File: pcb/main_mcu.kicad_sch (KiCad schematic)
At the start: 16 parts, among them U3 STM32H563VITx

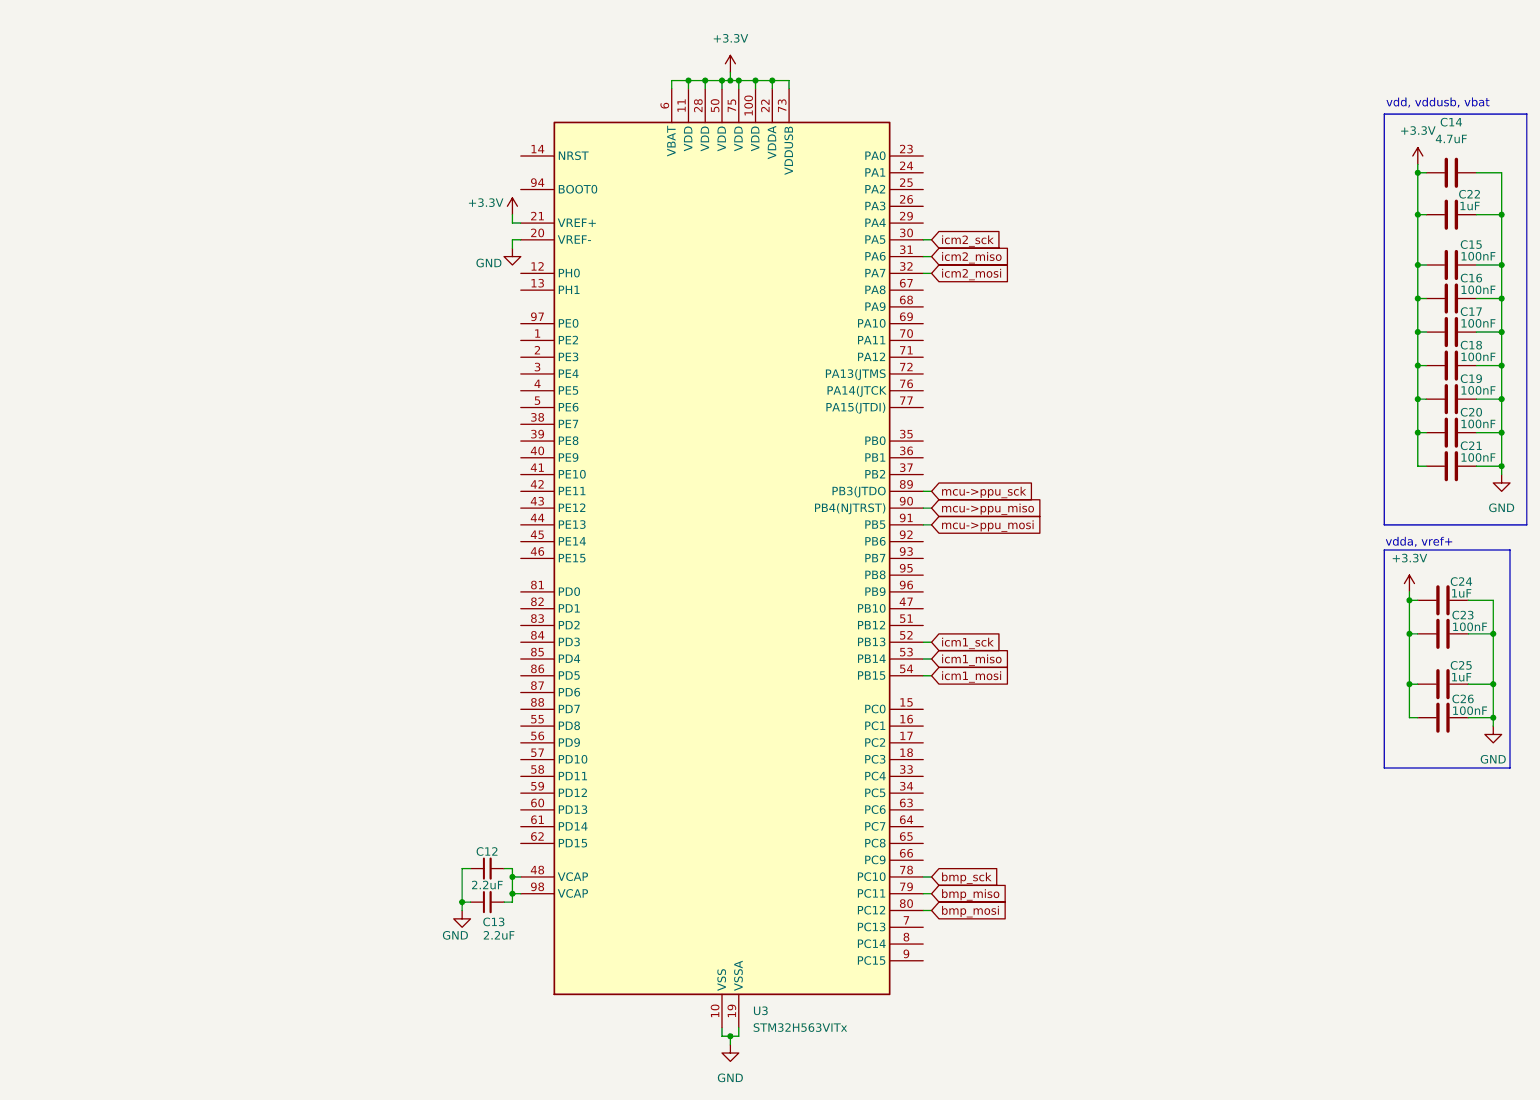
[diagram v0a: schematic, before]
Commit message: tons of work on rf and mcu
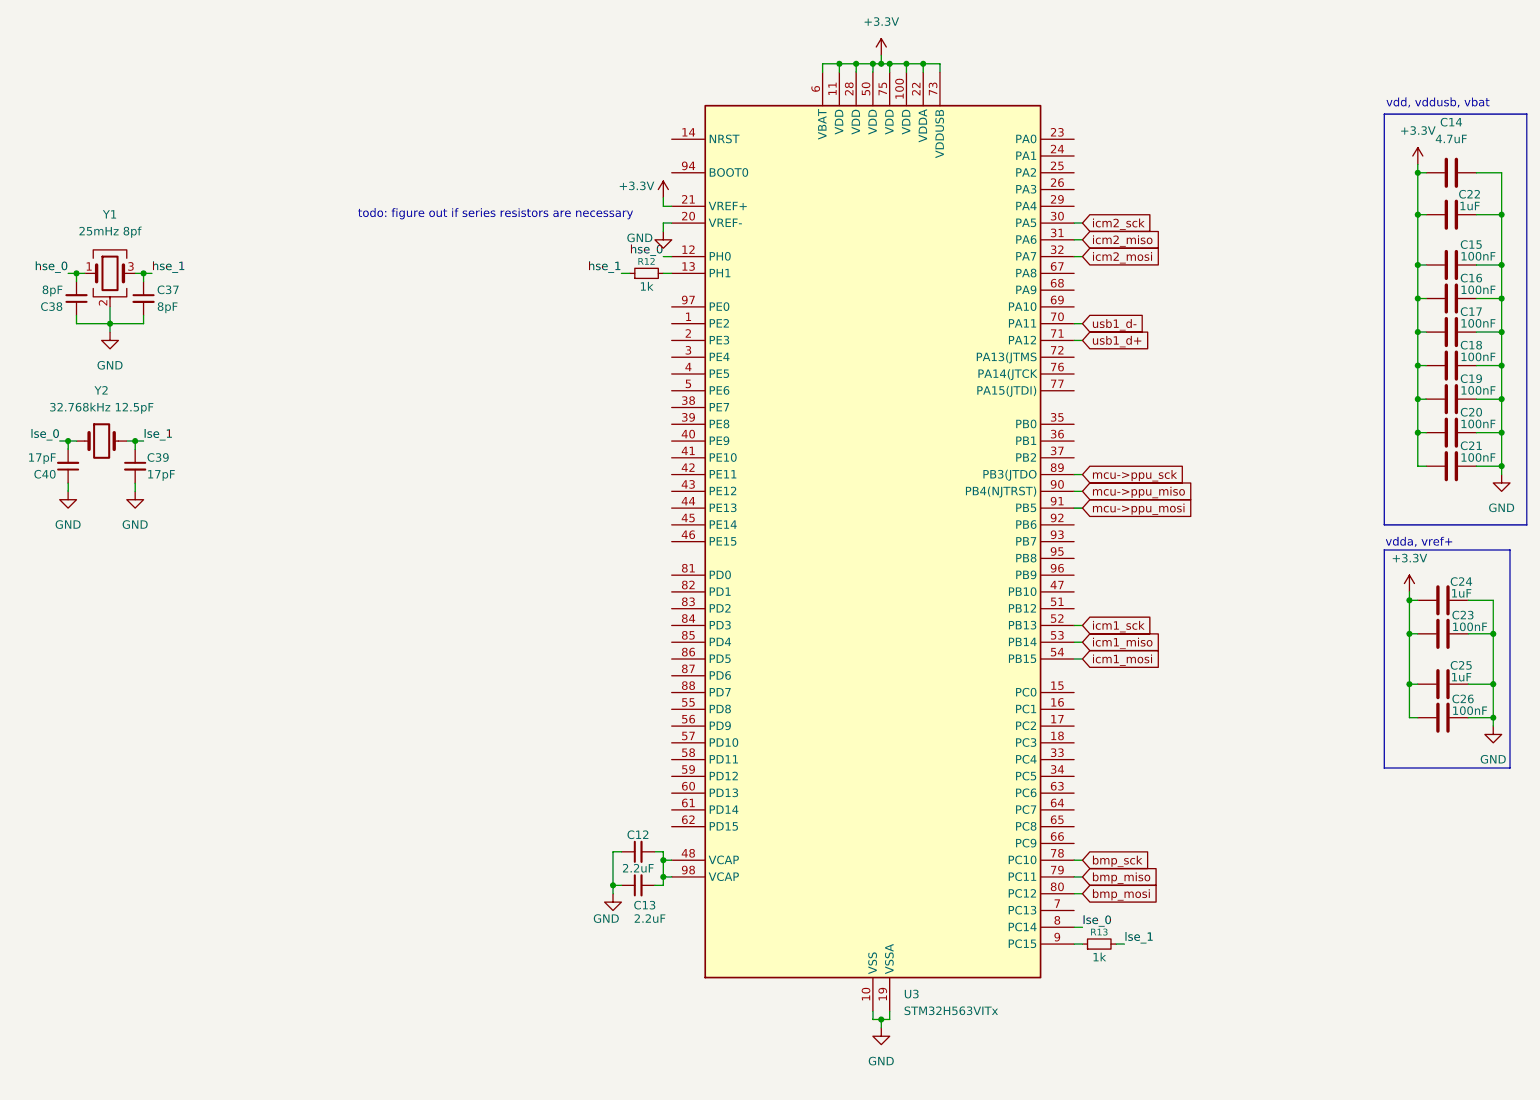
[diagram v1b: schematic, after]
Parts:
- added C37, C38: 8pF, symbol Device:C_Small
- added C39, C40: 17pF, symbol Device:C_Small
- added R12, R13: 1k, symbol Device:R_Small
- added Y1: 25mHz 8pf, symbol Device:Crystal_GND24
- added Y2: 32.768kHz 12.5pF, symbol Device:Crystal
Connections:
- net GND: now also C37.2, C38.1, C39.2, C40.1, Y1.2 (G), Y1.4 (G)
- net hse_0: now reaches U3.12 (PH0)
- net hse_0: now also C38.2, Y1.1
- net at U3.13 (PH1): now also R12.2
- net usb1_d-: now reaches U3.70 (PA11)
- net usb1_d+: now reaches U3.71 (PA12)
- net lse_0: now reaches U3.8 (PC14)
- net lse_0: now also C40.2, Y2.1
- net at U3.9 (PC15): now also R13.1
- new net hse_1: C37.1, R12.1, Y1.3
- new net lse_1: C39.1, R13.2, Y2.2
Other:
- note added: "todo: figure out if series resistors are necessary"
- moved on the sheet: C12, C13, U3

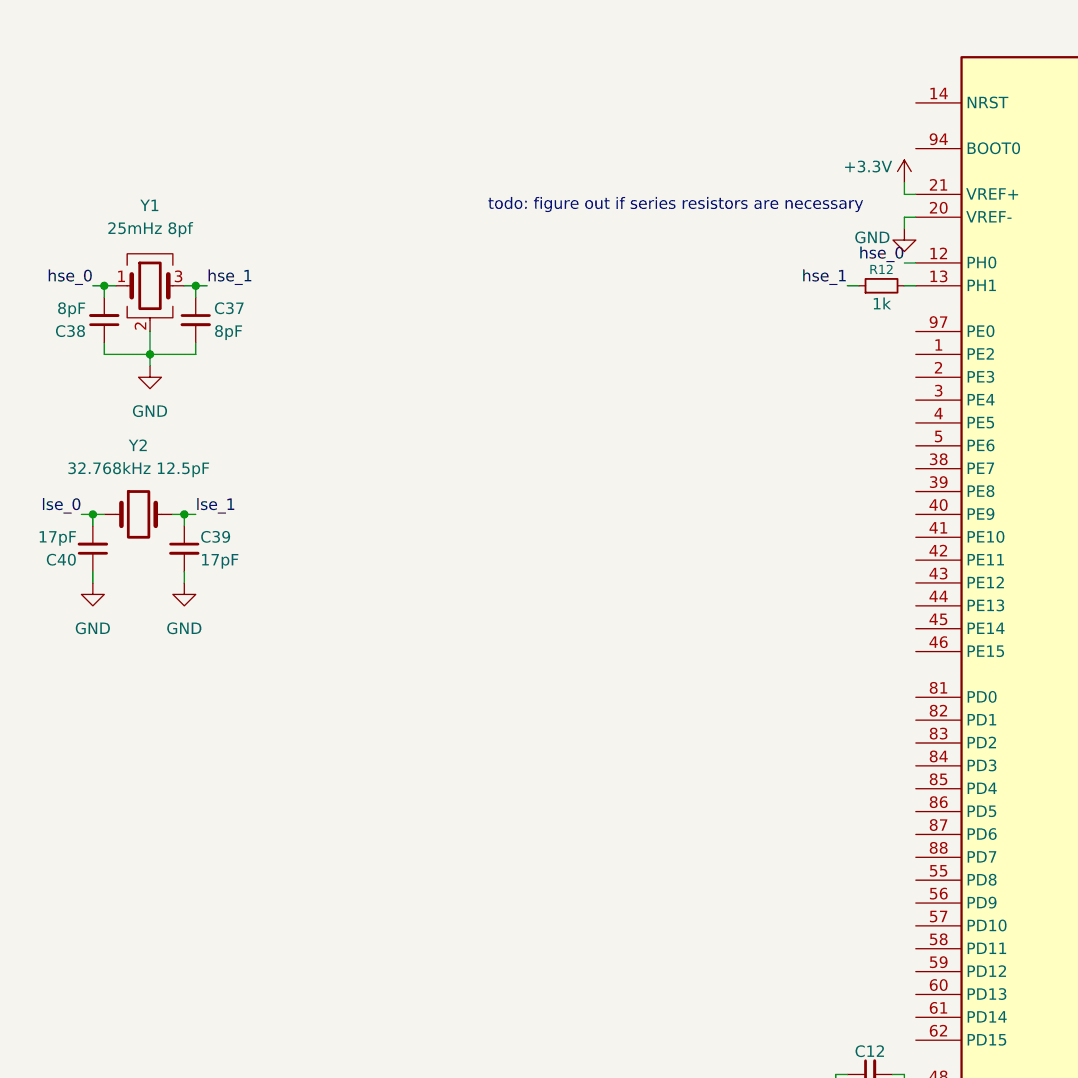
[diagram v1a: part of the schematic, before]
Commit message: added missing files, rf stuff done I think (hope)
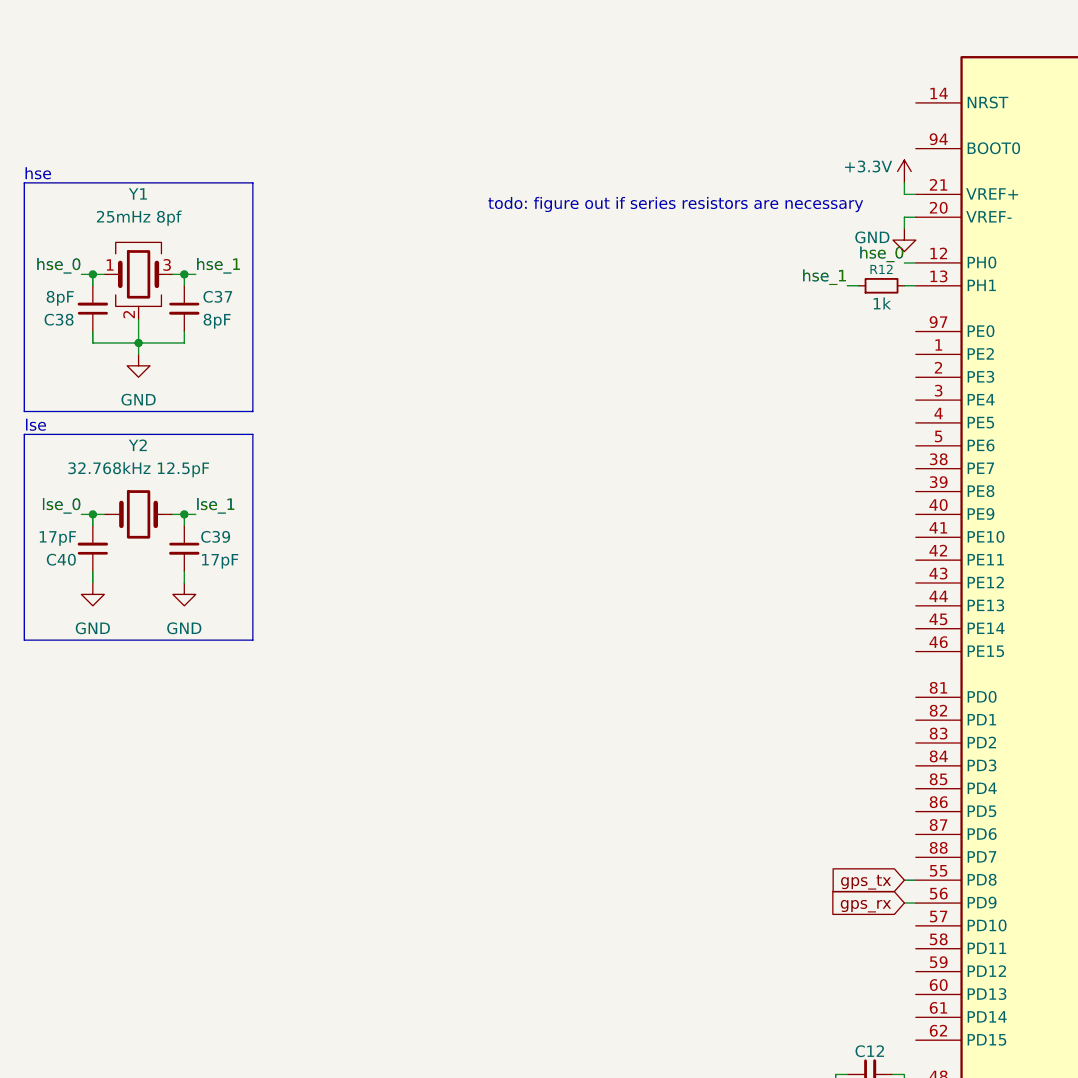
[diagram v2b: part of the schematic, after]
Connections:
- net gps_tx: now reaches U3.55 (PD8)
- net gps_rx: now reaches U3.56 (PD9)
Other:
- note added: "hse"
- note added: "lse"
- moved on the sheet: C37, C38, Y1
